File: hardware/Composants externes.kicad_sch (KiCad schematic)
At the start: 0 parts

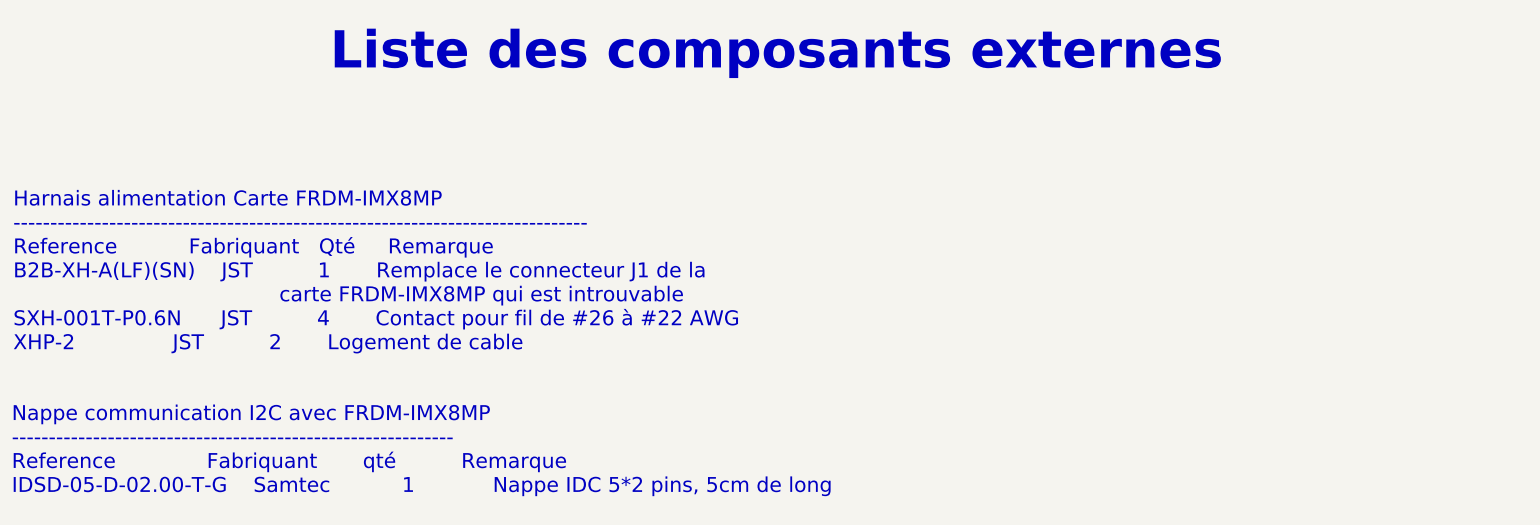
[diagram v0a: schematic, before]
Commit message: Erreur de manipulation, version 2.3 ok
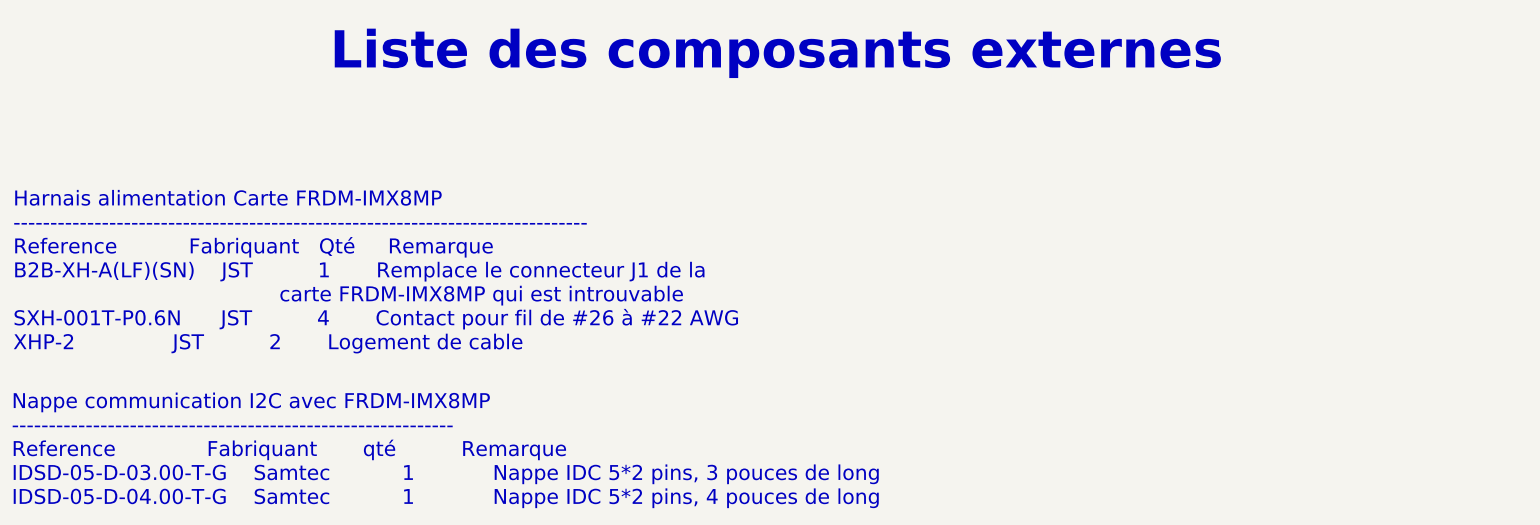
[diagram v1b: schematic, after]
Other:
- note added: "Nappe communication I2C avec FRDM-IMX8MP ------------------------------------------------------------ Reference Fabriquant qté Remarque IDSD-05-D-03.00-T-G Samtec 1 Nappe IDC 5*2 pins, 3 pouces de long IDSD-05-D-04.00-T-G Samtec 1 Nappe IDC 5*2 pins, 4 pouces de long"
- note removed: "Nappe communication I2C avec FRDM-IMX8MP ------------------------------------------------------------ Reference Fabriquant qté Remarque IDSD-05-D-02.00-T-G Samtec 1 Nappe IDC 5*2 pins, 5cm de long"
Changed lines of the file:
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@@
 		)
 	)
-	(text "Nappe communication I2C avec FRDM-IMX8MP\n------------------------------------------------------------\nReference              Fabriquant       qté          Remarque\nIDSD-05-D-02.00-T-G    Samtec           1            Nappe IDC 5*2 pins, 5cm de long"
+	(text "Nappe communication I2C avec FRDM-IMX8MP\n------------------------------------------------------------\nReference              Fabriquant       qté          Remarque\nIDSD-05-D-03.00-T-G    Samtec           1            Nappe IDC 5*2 pins, 3 pouces de long\nIDSD-05-D-04.00-T-G    Samtec           1            Nappe IDC 5*2 pins, 4 pouces de long"
 		(exclude_from_sim no)
 		(at 19.304 99.568 0)
